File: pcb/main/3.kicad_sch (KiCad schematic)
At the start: 10 parts

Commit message: fix: symbol libraries in Kicad 6.0
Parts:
- C19: value (none) -> 10u; footprint (none) -> Capacitor_SMD:C_0805_2012Metric_Pad1.15x1.40mm_HandSolder; symbol pHMeter-rescue:C-Device -> Device:C
- C22: value (none) -> 100n; footprint (none) -> Capacitor_SMD:C_0805_2012Metric_Pad1.15x1.40mm_HandSolder; symbol pHMeter-rescue:C-Device -> Device:C
- C24, C25: value (none) -> 22u; footprint (none) -> Capacitor_SMD:C_0805_2012Metric_Pad1.15x1.40mm_HandSolder; symbol pHMeter-rescue:C-Device -> Device:C
- D15, D16: value (none) -> GREEN; footprint (none) -> LED_SMD:LED_0805_2012Metric_Pad1.15x1.40mm_HandSolder; symbol pHMeter-rescue:LED-Device -> Device:LED
- L2: symbol pHMeter-rescue:L-Device -> Device:L
- R39: renamed from R?; value (none) -> 10k; footprint (none) -> Resistor_SMD:R_0805_2012Metric_Pad1.15x1.40mm_HandSolder; symbol pHMeter-rescue:R-Device -> Device:R
- R40: renamed from R?; value (none) -> 1k; footprint (none) -> Resistor_SMD:R_0805_2012Metric_Pad1.15x1.40mm_HandSolder; symbol pHMeter-rescue:R-Device -> Device:R
- U5: value (none) -> AP63203WU-7; footprint (none) -> Package_TO_SOT_SMD:TSOT-23-6
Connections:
- net 3.3V: now also C24.2, C25.2, L2.2, R40.1
- net GND: now also C19.2, C24.1, C25.1, D15.1 (K), D16.1 (K)
- net VIN: now also C19.1, R39.1
- net at U5.5 (SW): now also C22.1, L2.1
- net at U5.6 (BST): now also C22.2
- new net: D15.2 (A), R39.2
- new net: D16.2 (A), R40.2
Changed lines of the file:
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@@
     (effects (font (size 1.27 1.27)) (justify right))
   )
-  (symbol (lib_id "pHMeter-rescue:R-Device") (at 173.99 95.885 0) (unit 1)
-    (in_bom yes) (on_board yes)
-    (property "Reference" "R?" (id 0) (at 172.085 95.885 90))
-    (property "Value" "" (id 1) (at 173.99 95.885 90))
-    (property "Footprint" "" (id 2) (at 172.212 95.885 90)
+  (symbol (lib_id "Device:R") (at 173.99 95.885 0) (unit 1)
+    (in_bom yes) (on_board yes)
+    (property "Reference" "R39" (id 0) (at 172.085 95.885 90))
+    (property "Value" "10k" (id 1) (at 173.99 95.885 90))
+    (property "Footprint" "Resistor_SMD:R_0805_2012Metric_Pad1.15x1.40mm_HandSolder" (id 2) (at 172.212 95.885 90)
       (effects (font (size 1.27 1.27)) hide)
     )
@@
       (effects (font (size 1.27 1.27)) hide)
     )
-  )
-  (symbol (lib_id "pHMeter-rescue:R-Device") (at 189.23 95.885 0) (unit 1)
-    (in_bom yes) (on_board yes)
-    (property "Reference" "R?" (id 0) (at 187.325 95.885 90))
-    (property "Value" "" (id 1) (at 189.23 95.885 90))
-    (property "Footprint" "" (id 2) (at 187.452 95.885 90)
+    (pin "1")
+    (pin "2")
+  )
+  (symbol (lib_id "Device:R") (at 189.23 95.885 0) (unit 1)
+    (in_bom yes) (on_board yes)
+    (property "Reference" "R40" (id 0) (at 187.325 95.885 90))
+    (property "Value" "1k" (id 1) (at 189.23 95.885 90))
+    (property "Footprint" "Resistor_SMD:R_0805_2012Metric_Pad1.15x1.40mm_HandSolder" (id 2) (at 187.452 95.885 90)
       (effects (font (size 1.27 1.27)) hide)
     )
@@
       (effects (font (size 1.27 1.27)) hide)
     )
-  )
-  (symbol (lib_id "pHMeter-rescue:LED-Device") (at 173.99 106.045 270) (mirror x) (unit 1)
+    (pin "1")
+    (pin "2")
+  )
+  (symbol (lib_id "Device:LED") (at 173.99 106.045 270) (mirror x) (unit 1)
     (in_bom yes) (on_board yes)
     (property "Reference" "D15" (id 0) (at 172.085 106.045 0))
-    (property "Value" "" (id 1) (at 176.53 106.045 0))
-    (property "Footprint" "" (id 2) (at 173.99 106.045 0)
+    (property "Value" "GREEN" (id 1) (at 176.53 106.045 0))
+    (property "Footprint" "LED_SMD:LED_0805_2012Metric_Pad1.15x1.40mm_HandSolder" (id 2) (at 173.99 106.045 0)
       (effects (font (size 1.27 1.27)) hide)
     )
@@
       (effects (font (size 1.27 1.27)) hide)
     )
-  )
-  (symbol (lib_id "pHMeter-rescue:LED-Device") (at 189.23 106.045 270) (mirror x) (unit 1)
+    (pin "1")
+    (pin "2")
+  )
+  (symbol (lib_id "Device:LED") (at 189.23 106.045 270) (mirror x) (unit 1)
     (in_bom yes) (on_board yes)
     (property "Reference" "D16" (id 0) (at 187.325 106.045 0))
-    (property "Value" "" (id 1) (at 191.77 106.045 0))
-    (property "Footprint" "" (id 2) (at 189.23 106.045 0)
+    (property "Value" "GREEN" (id 1) (at 191.77 106.045 0))
+    (property "Footprint" "LED_SMD:LED_0805_2012Metric_Pad1.15x1.40mm_HandSolder" (id 2) (at 189.23 106.045 0)
       (effects (font (size 1.27 1.27)) hide)
     )
@@
       (effects (font (size 1.27 1.27)) hide)
     )
+    (pin "1")
+    (pin "2")
   )
   (symbol (lib_id "bioreactor:AP63203WU-7") (at 103.505 97.79 0) (unit 1)
     (in_bom yes) (on_board yes)
     (property "Reference" "U5" (id 0) (at 103.505 88.4682 0))
-    (property "Value" "" (id 1) (at 103.505 90.7796 0))
-    (property "Footprint" "" (id 2) (at 103.505 120.65 0)
+    (property "Value" "AP63203WU-7" (id 1) (at 103.505 90.7796 0))
+    (property "Footprint" "Package_TO_SOT_SMD:TSOT-23-6" (id 2) (at 103.505 120.65 0)
       (effects (font (size 1.27 1.27)) hide)
     )
@@
     (pin "6")
   )
-  (symbol (lib_id "pHMeter-rescue:C-Device") (at 85.09 100.33 0) (unit 1)
+  (symbol (lib_id "Device:C") (at 85.09 100.33 0) (unit 1)
     (in_bom yes) (on_board yes)
     (property "Reference" "C19" (id 0) (at 88.011 99.1616 0)
       (effects (font (size 1.27 1.27)) (justify left))
     )
-    (property "Value" "" (id 1) (at 88.011 101.473 0)
+    (property "Value" "10u" (id 1) (at 88.011 101.473 0)
       (effects (font (size 1.27 1.27)) (justify left))
     )
-    (property "Footprint" "" (id 2) (at 86.0552 104.14 0)
+    (property "Footprint" "Capacitor_SMD:C_0805_2012Metric_Pad1.15x1.40mm_HandSolder" (id 2) (at 86.0552 104.14 0)
       (effects (font (size 1.27 1.27)) hide)
     )
@@
       (effects (font (size 1.27 1.27)) hide)
     )
-  )
-  (symbol (lib_id "pHMeter-rescue:C-Device") (at 119.38 97.79 270) (unit 1)
+    (pin "1")
+    (pin "2")
+  )
+  (symbol (lib_id "Device:C") (at 119.38 97.79 270) (unit 1)
     (in_bom yes) (on_board yes)
     (property "Reference" "C22" (id 0) (at 119.38 91.3892 90))
-    (property "Value" "" (id 1) (at 119.38 93.7006 90))
-    (property "Footprint" "" (id 2) (at 115.57 98.7552 0)
+    (property "Value" "100n" (id 1) (at 119.38 93.7006 90))
+    (property "Footprint" "Capacitor_SMD:C_0805_2012Metric_Pad1.15x1.40mm_HandSolder" (id 2) (at 115.57 98.7552 0)
       (effects (font (size 1.27 1.27)) hide)
     )
@@
       (effects (font (size 1.27 1.27)) hide)
     )
-  )
-  (symbol (lib_id "pHMeter-rescue:L-Device") (at 130.175 95.25 90) (unit 1)
+    (pin "1")
+    (pin "2")
+  )
+  (symbol (lib_id "Device:L") (at 130.175 95.25 90) (unit 1)
     (in_bom yes) (on_board yes)
     (property "Reference" "L2" (id 0) (at 130.175 90.424 90))
@@
       (effects (font (size 1.27 1.27)) hide)
     )
-  )
-  (symbol (lib_id "pHMeter-rescue:C-Device") (at 138.43 100.33 180) (unit 1)
+    (pin "1")
+    (pin "2")
+  )
+  (symbol (lib_id "Device:C") (at 138.43 100.33 180) (unit 1)
     (in_bom yes) (on_board yes)
     (property "Reference" "C24" (id 0) (at 141.351 99.1616 0)
       (effects (font (size 1.27 1.27)) (justify right))
     )
-    (property "Value" "" (id 1) (at 141.351 101.473 0)
-      (effects (font (size 1.27 1.27)) (justify right))
-    )
-    (property "Footprint" "" (id 2) (at 137.4648 96.52 0)
+    (property "Value" "22u" (id 1) (at 141.351 101.473 0)
+      (effects (font (size 1.27 1.27)) (justify right))
+    )
+    (property "Footprint" "Capacitor_SMD:C_0805_2012Metric_Pad1.15x1.40mm_HandSolder" (id 2) (at 137.4648 96.52 0)
       (effects (font (size 1.27 1.27)) hide)
     )
@@
       (effects (font (size 1.27 1.27)) hide)
     )
-  )
-  (symbol (lib_id "pHMeter-rescue:C-Device") (at 147.32 100.33 180) (unit 1)
+    (pin "1")
+    (pin "2")
+  )
+  (symbol (lib_id "Device:C") (at 147.32 100.33 180) (unit 1)
     (in_bom yes) (on_board yes)
     (property "Reference" "C25" (id 0) (at 150.241 99.1616 0)
       (effects (font (size 1.27 1.27)) (justify right))
     )
-    (property "Value" "" (id 1) (at 150.241 101.473 0)
-      (effects (font (size 1.27 1.27)) (justify right))
-    )
-    (property "Footprint" "" (id 2) (at 146.3548 96.52 0)
+    (property "Value" "22u" (id 1) (at 150.241 101.473 0)
+      (effects (font (size 1.27 1.27)) (justify right))
+    )
+    (property "Footprint" "Capacitor_SMD:C_0805_2012Metric_Pad1.15x1.40mm_HandSolder" (id 2) (at 146.3548 96.52 0)
       (effects (font (size 1.27 1.27)) hide)
     )
@@
       (effects (font (size 1.27 1.27)) hide)
     )
+    (pin "1")
+    (pin "2")
   )
 )

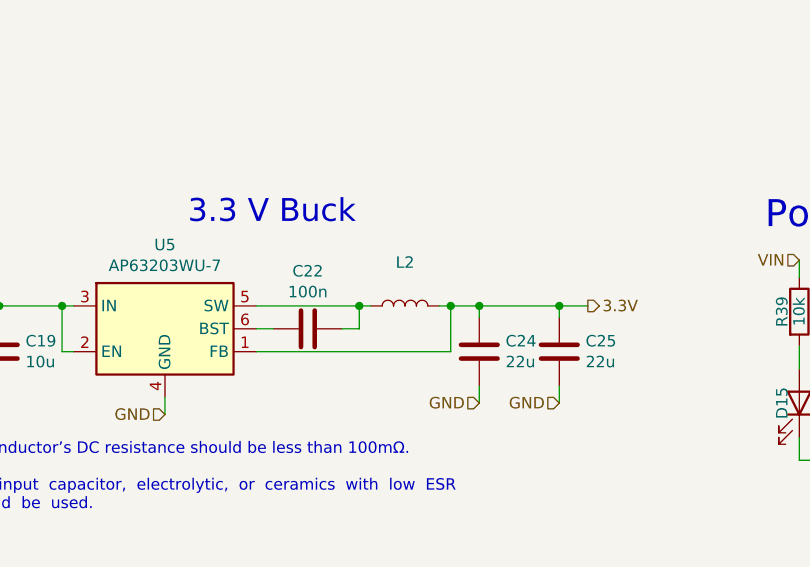
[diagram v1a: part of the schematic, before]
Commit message: fix: 3D model libraries in Kicad 6.0
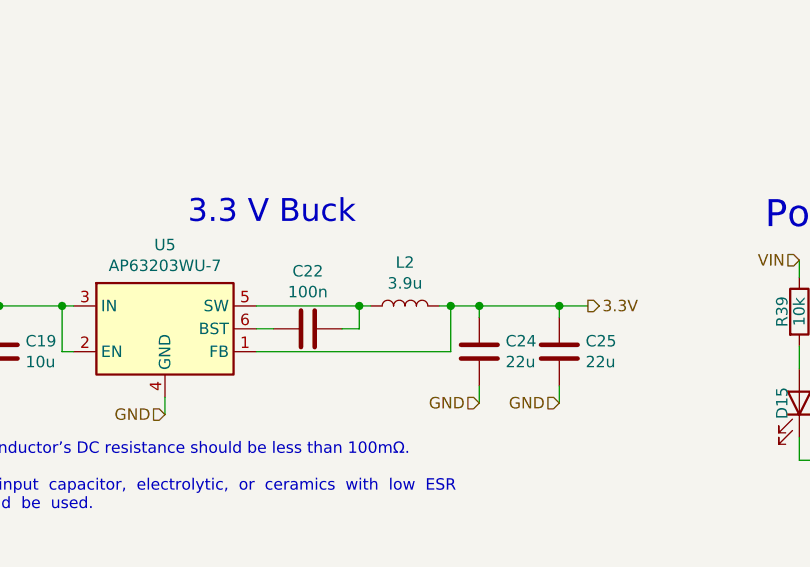
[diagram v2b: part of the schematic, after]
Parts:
- L2: value (none) -> 3.9u; footprint (none) -> Inductor_SMD:L_Taiyo-Yuden_NR-24xx_HandSoldering
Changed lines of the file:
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@@
     (in_bom yes) (on_board yes)
     (property "Reference" "L2" (id 0) (at 130.175 90.424 90))
-    (property "Value" "" (id 1) (at 130.175 92.7354 90))
-    (property "Footprint" "" (id 2) (at 130.175 95.25 0)
+    (property "Value" "3.9u" (id 1) (at 130.175 92.7354 90))
+    (property "Footprint" "Inductor_SMD:L_Taiyo-Yuden_NR-24xx_HandSoldering" (id 2) (at 130.175 95.25 0)
       (effects (font (size 1.27 1.27)) hide)
     )

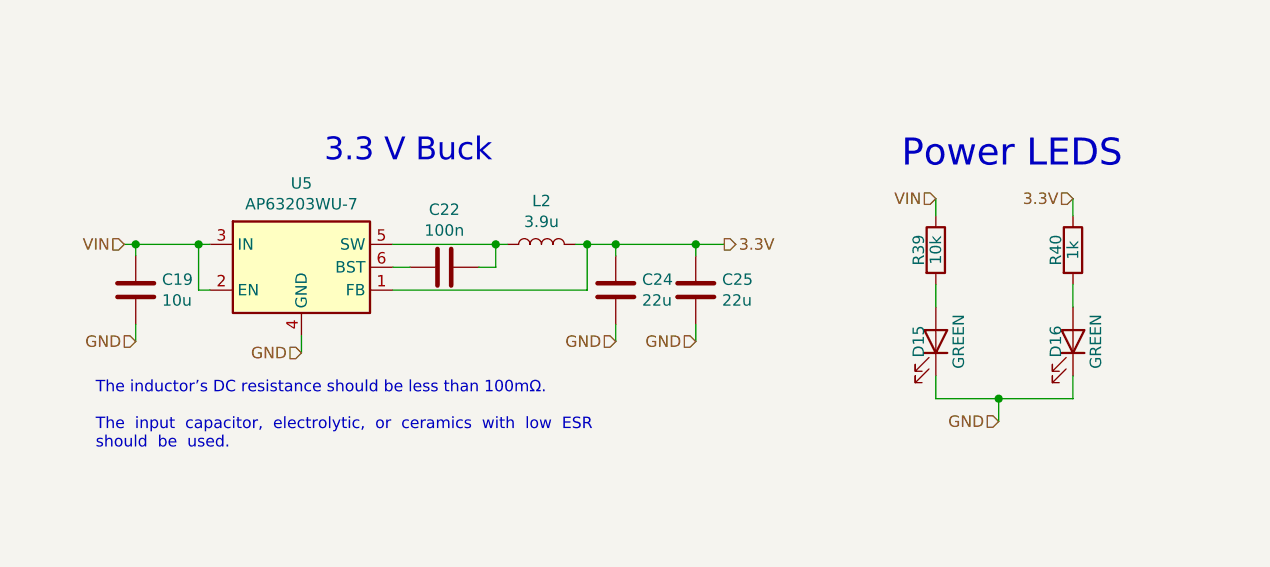
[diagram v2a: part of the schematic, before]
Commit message: fix: standard footprint for R and C, BOM updated
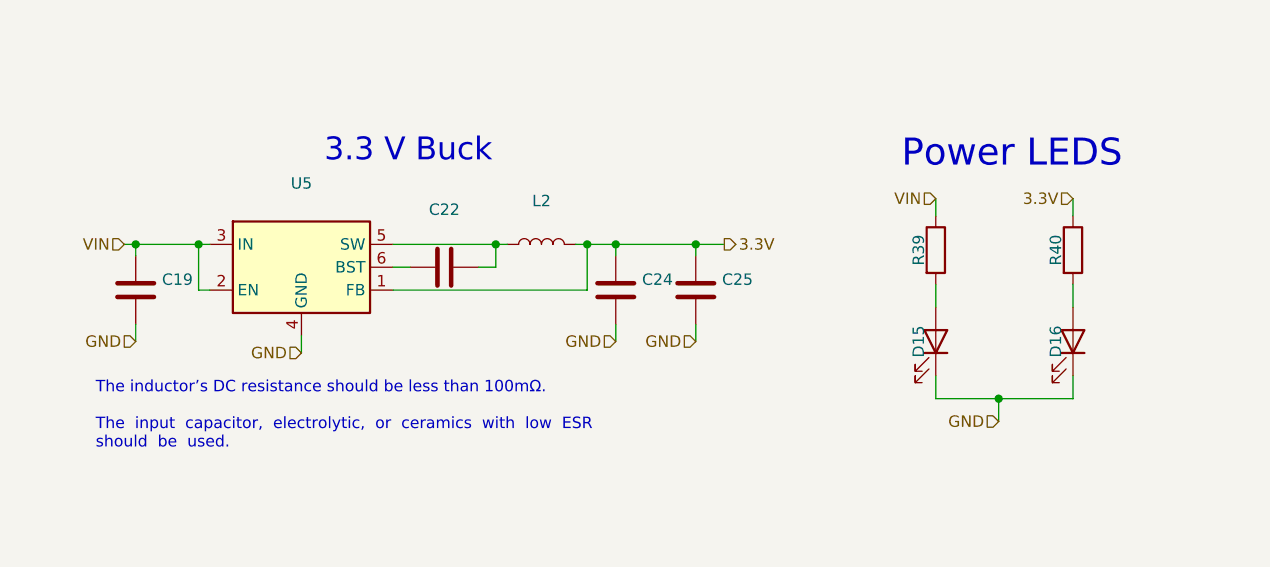
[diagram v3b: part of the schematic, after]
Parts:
- C19: value 10u -> (none); footprint Capacitor_SMD:C_0805_2012Metric_Pad1.15x1.40mm_HandSolder -> (none); MFN Samsung Electro-Mechanics -> Wurth Elektronik; MFP CL21A106KOQNNNG -> 885012207072; S1PL https://www.mouser.com/ProductDetail/Samsung-Electro-Mechan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 -> https://www.mouser.com/ProductDetail/Wurth-Elektronik/88501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; S1PN 187-CL21A106KOQNNNG -> 710-885012207072
- C22: value 100n -> (none); footprint Capacitor_SMD:C_0805_2012Metric_Pad1.15x1.40mm_HandSolder -> (none)
- C24, C25: value 22u -> (none); footprint Capacitor_SMD:C_0805_2012Metric_Pad1.15x1.40mm_HandSolder -> (none)
- D15, D16: value GREEN -> (none); footprint LED_SMD:LED_0805_2012Metric_Pad1.15x1.40mm_HandSolder -> (none)
- L2: value 3.9u -> (none); footprint Inductor_SMD:L_Taiyo-Yuden_NR-24xx_HandSoldering -> (none)
- R39: value 10k -> (none); footprint Resistor_SMD:R_0805_2012Metric_Pad1.15x1.40mm_HandSolder -> (none)
- R40: value 1k -> (none); footprint Resistor_SMD:R_0805_2012Metric_Pad1.15x1.40mm_HandSolder -> (none)
- U5: value AP63203WU-7 -> (none); footprint Package_TO_SOT_SMD:TSOT-23-6 -> (none)
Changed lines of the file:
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@@
     (in_bom yes) (on_board yes)
     (property "Reference" "R39" (id 0) (at 172.085 95.885 90))
-    (property "Value" "10k" (id 1) (at 173.99 95.885 90))
-    (property "Footprint" "Resistor_SMD:R_0805_2012Metric_Pad1.15x1.40mm_HandSolder" (id 2) (at 172.212 95.885 90)
+    (property "Value" "" (id 1) (at 173.99 95.885 90))
+    (property "Footprint" "" (id 2) (at 172.212 95.885 90)
       (effects (font (size 1.27 1.27)) hide)
     )
@@
     (in_bom yes) (on_board yes)
     (property "Reference" "R40" (id 0) (at 187.325 95.885 90))
-    (property "Value" "1k" (id 1) (at 189.23 95.885 90))
-    (property "Footprint" "Resistor_SMD:R_0805_2012Metric_Pad1.15x1.40mm_HandSolder" (id 2) (at 187.452 95.885 90)
+    (property "Value" "" (id 1) (at 189.23 95.885 90))
+    (property "Footprint" "" (id 2) (at 187.452 95.885 90)
       (effects (font (size 1.27 1.27)) hide)
     )
@@
     (in_bom yes) (on_board yes)
     (property "Reference" "D15" (id 0) (at 172.085 106.045 0))
-    (property "Value" "GREEN" (id 1) (at 176.53 106.045 0))
-    (property "Footprint" "LED_SMD:LED_0805_2012Metric_Pad1.15x1.40mm_HandSolder" (id 2) (at 173.99 106.045 0)
+    (property "Value" "" (id 1) (at 176.53 106.045 0))
+    (property "Footprint" "" (id 2) (at 173.99 106.045 0)
       (effects (font (size 1.27 1.27)) hide)
     )
@@
     (in_bom yes) (on_board yes)
     (property "Reference" "D16" (id 0) (at 187.325 106.045 0))
-    (property "Value" "GREEN" (id 1) (at 191.77 106.045 0))
-    (property "Footprint" "LED_SMD:LED_0805_2012Metric_Pad1.15x1.40mm_HandSolder" (id 2) (at 189.23 106.045 0)
+    (property "Value" "" (id 1) (at 191.77 106.045 0))
+    (property "Footprint" "" (id 2) (at 189.23 106.045 0)
       (effects (font (size 1.27 1.27)) hide)
     )
@@
     (in_bom yes) (on_board yes)
     (property "Reference" "U5" (id 0) (at 103.505 88.4682 0))
-    (property "Value" "AP63203WU-7" (id 1) (at 103.505 90.7796 0))
-    (property "Footprint" "Package_TO_SOT_SMD:TSOT-23-6" (id 2) (at 103.505 120.65 0)
+    (property "Value" "" (id 1) (at 103.505 90.7796 0))
+    (property "Footprint" "" (id 2) (at 103.505 120.65 0)
       (effects (font (size 1.27 1.27)) hide)
     )
@@
       (effects (font (size 1.27 1.27)) (justify left))
     )
-    (property "Value" "10u" (id 1) (at 88.011 101.473 0)
+    (property "Value" "" (id 1) (at 88.011 101.473 0)
       (effects (font (size 1.27 1.27)) (justify left))
     )
-    (property "Footprint" "Capacitor_SMD:C_0805_2012Metric_Pad1.15x1.40mm_HandSolder" (id 2) (at 86.0552 104.14 0)
-      (effects (font (size 1.27 1.27)) hide)
-    )
-    (property "Datasheet" "https://www.mouser.com/datasheet/2/585/MLCC-1837944.pdf" (id 3) (at 85.09 100.33 0)
-      (effects (font (size 1.27 1.27)) hide)
-    )
-    (property "Description" "Multilayer Ceramic Capacitors MLCC - SMD/SMT 16V 10uF X5R 0805 10%" (id 4) (at 85.09 100.33 0)
-      (effects (font (size 1.27 1.27)) hide)
-    )
-    (property "MFN" "Samsung Electro-Mechanics " (id 5) (at 85.09 100.33 0)
-      (effects (font (size 1.27 1.27)) hide)
-    )
-    (property "MFP" "CL21A106KOQNNNG " (id 6) (at 85.09 100.33 0)
-      (effects (font (size 1.27 1.27)) hide)
-    )
-    (property "S1PL" "https://www.mouser.com/ProductDetail/Samsung-Electro-Mechanics/CL21A106KOQNNNG?qs=hqM3L16%252BxlcMWI7QbqH0LA%3D%3D" (id 7) (at 85.09 100.33 0)
-      (effects (font (size 1.27 1.27)) hide)
-    )
-    (property "S1PN" " 187-CL21A106KOQNNNG " (id 8) (at 85.09 100.33 0)
+    (property "Footprint" "" (id 2) (at 86.0552 104.14 0)
+      (effects (font (size 1.27 1.27)) hide)
+    )
+    (property "Datasheet" "https://www.mouser.com/datasheet/2/445/885012207072-1727745.pdf" (id 3) (at 85.09 100.33 0)
+      (effects (font (size 1.27 1.27)) hide)
+    )
+    (property "Description" "Multilayer Ceramic Capacitors MLCC - SMD/SMT WCAP-CSGP 0.1uF 0805 10% 25V MLCC " (id 4) (at 85.09 100.33 0)
+      (effects (font (size 1.27 1.27)) hide)
+    )
+    (property "MFN" "Wurth Elektronik " (id 5) (at 85.09 100.33 0)
+      (effects (font (size 1.27 1.27)) hide)
+    )
+    (property "MFP" "885012207072" (id 6) (at 85.09 100.33 0)
+      (effects (font (size 1.27 1.27)) hide)
+    )
+    (property "S1PL" "https://www.mouser.com/ProductDetail/Wurth-Elektronik/885012207072?qs=0KOYDY2FL28rQMV4504TxA%3D%3D" (id 7) (at 85.09 100.33 0)
+      (effects (font (size 1.27 1.27)) hide)
+    )
+    (property "S1PN" "710-885012207072 " (id 8) (at 85.09 100.33 0)
       (effects (font (size 1.27 1.27)) hide)
     )
@@
     (in_bom yes) (on_board yes)
     (property "Reference" "C22" (id 0) (at 119.38 91.3892 90))
-    (property "Value" "100n" (id 1) (at 119.38 93.7006 90))
-    (property "Footprint" "Capacitor_SMD:C_0805_2012Metric_Pad1.15x1.40mm_HandSolder" (id 2) (at 115.57 98.7552 0)
+    (property "Value" "" (id 1) (at 119.38 93.7006 90))
+    (property "Footprint" "" (id 2) (at 115.57 98.7552 0)
       (effects (font (size 1.27 1.27)) hide)
     )
@@
     (in_bom yes) (on_board yes)
     (property "Reference" "L2" (id 0) (at 130.175 90.424 90))
-    (property "Value" "3.9u" (id 1) (at 130.175 92.7354 90))
-    (property "Footprint" "Inductor_SMD:L_Taiyo-Yuden_NR-24xx_HandSoldering" (id 2) (at 130.175 95.25 0)
+    (property "Value" "" (id 1) (at 130.175 92.7354 90))
+    (property "Footprint" "" (id 2) (at 130.175 95.25 0)
       (effects (font (size 1.27 1.27)) hide)
     )
@@
       (effects (font (size 1.27 1.27)) (justify right))
     )
-    (property "Value" "22u" (id 1) (at 141.351 101.473 0)
-      (effects (font (size 1.27 1.27)) (justify right))
-    )
-    (property "Footprint" "Capacitor_SMD:C_0805_2012Metric_Pad1.15x1.40mm_HandSolder" (id 2) (at 137.4648 96.52 0)
+    (property "Value" "" (id 1) (at 141.351 101.473 0)
+      (effects (font (size 1.27 1.27)) (justify right))
+    )
+    (property "Footprint" "" (id 2) (at 137.4648 96.52 0)
       (effects (font (size 1.27 1.27)) hide)
     )
@@
       (effects (font (size 1.27 1.27)) (justify right))
     )
-    (property "Value" "22u" (id 1) (at 150.241 101.473 0)
-      (effects (font (size 1.27 1.27)) (justify right))
-    )
-    (property "Footprint" "Capacitor_SMD:C_0805_2012Metric_Pad1.15x1.40mm_HandSolder" (id 2) (at 146.3548 96.52 0)
-      (effects (font (size 1.27 1.27)) hide)
-    )
+    (property "Value" "" (id 1) (at 150.241 101.473 0)
+      (effects (font (size 1.27 1.27)) (justify right))
+    )
+    (property "Footprint" "" (id 2) (at 146.3548 96.52 0)
+      (effects (font (size 1.27 1.27)) hide)
+    )
